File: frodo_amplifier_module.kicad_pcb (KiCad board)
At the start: 2 copper layers, 16.5 x 21.2 mm, 23 parts, among them IC1 INA826AID, IC2 AS321KTR-G1, J1 Conn_01x01_Socket, J2 Conn_01x01_Socket, J3 Conn_01x01_Socket, J4 Conn_01x01_Socket, J5 Conn_01x01_Socket, J6 Conn_01x01_Socket, J7 Conn_01x01_Socket, J8 Conn_01x01_Socket

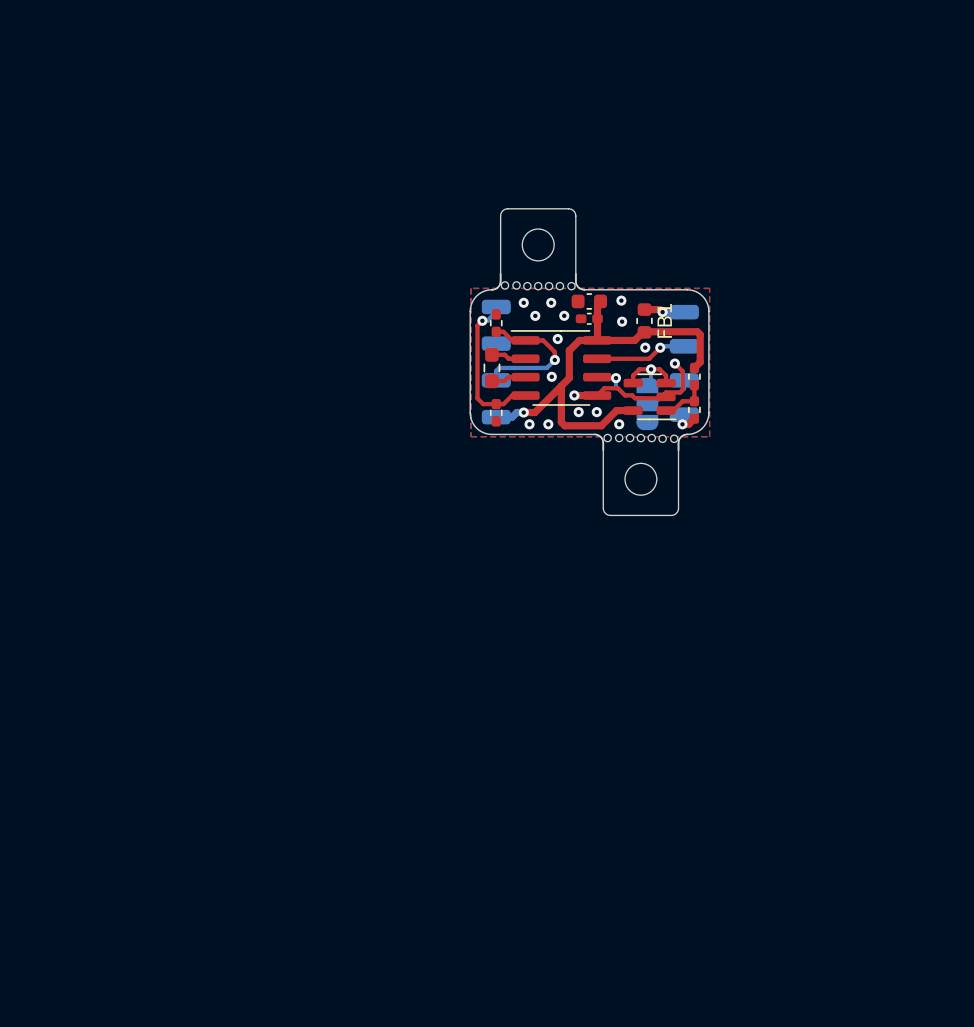
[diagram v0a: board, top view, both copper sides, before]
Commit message: finished the scematics
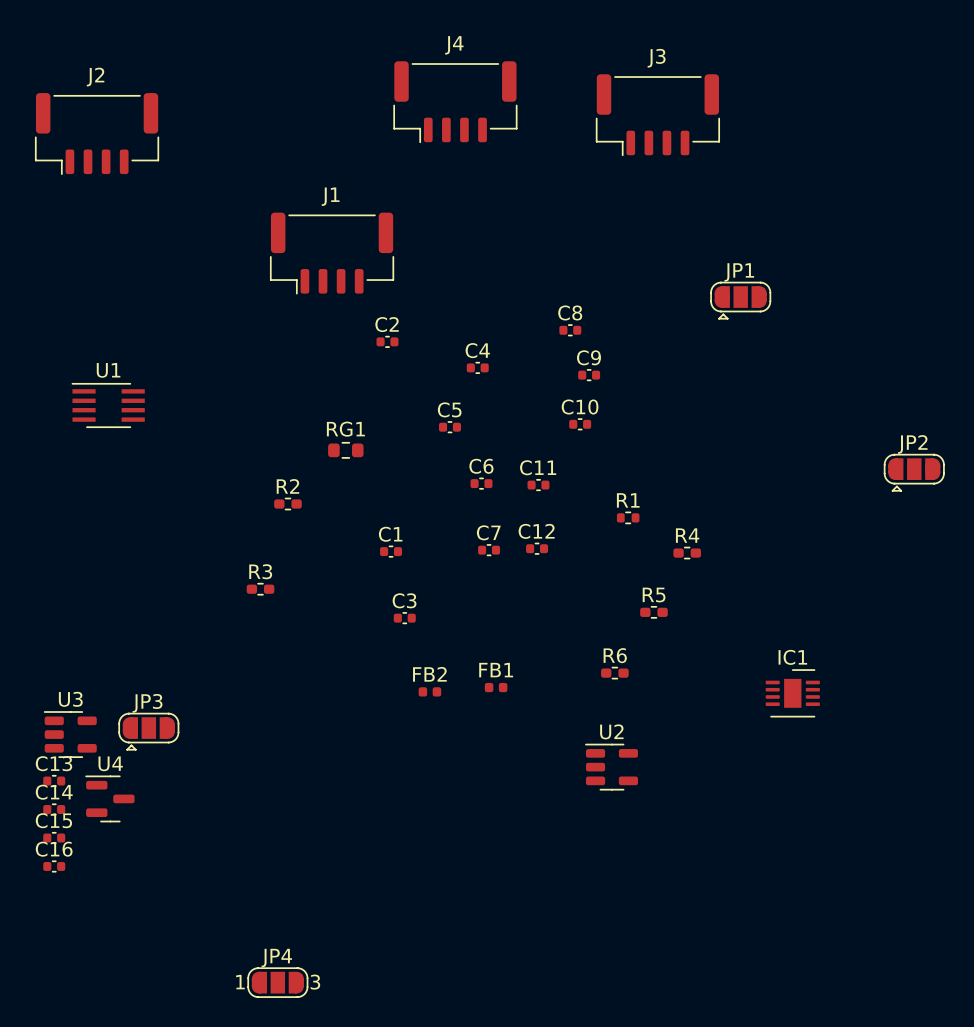
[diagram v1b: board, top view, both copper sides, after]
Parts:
- removed IC2: AS321KTR-G1, Package_TO_SOT_SMD:SOT-23-5
- removed J5, J6, J7, J8: Conn_01x01_Socket, Connector_Wire:SolderWirePad_1x01_SMD_1x2mm
- removed REF** (x2): MountingHole_2.2mm_M2, MountingHole:MountingHole_2.2mm_M2
- removed mouse-bite-2mm-slot (x2): VAL**, MountingEquipment:mouse-bite-2mm-slot
- added C10: 2n2, Capacitor_SMD:C_0402_1005Metric, F.Cu at (80.6, 55.3)
- added C11: 470n, Capacitor_SMD:C_0402_1005Metric, F.Cu at (77.7, 59.5)
- added C12: 0u1, Capacitor_SMD:C_0402_1005Metric, F.Cu at (77.6, 63.9)
- added C13: 0u1, Capacitor_SMD:C_0402_1005Metric, F.Cu at (44.2, 80.0)
- added C14: 0u1, Capacitor_SMD:C_0402_1005Metric, F.Cu at (44.2, 81.9)
- added C15: 1u, Capacitor_SMD:C_0402_1005Metric, F.Cu at (44.2, 83.9)
- added C16: 1u, Capacitor_SMD:C_0402_1005Metric, F.Cu at (44.2, 85.9)
- added C3: 4u7, Capacitor_SMD:C_0402_1005Metric, F.Cu at (68.5, 68.7)
- added C4: 0u1, Capacitor_SMD:C_0402_1005Metric, F.Cu at (73.5, 51.4)
- added C5: 10n, Capacitor_SMD:C_0402_1005Metric, F.Cu at (71.6, 55.5)
- added C6: 2n2, Capacitor_SMD:C_0402_1005Metric, F.Cu at (73.8, 59.4)
- added C7: 10n, Capacitor_SMD:C_0402_1005Metric, F.Cu at (74.3, 64.0)
- added C8: 10n, Capacitor_SMD:C_0402_1005Metric, F.Cu at (79.9, 48.8)
- added C9: 2n2, Capacitor_SMD:C_0402_1005Metric, F.Cu at (81.2, 51.9)
- added FB2: 120R, Inductor_SMD:L_0402_1005Metric, F.Cu at (70.2, 73.8)
- added JP2: SolderJumper_3_Open, Jumper:SolderJumper-3_P1.3mm_Open_RoundedPad1.0x1.5mm, F.Cu at (103.7, 58.4)
- added JP3: SolderJumper_3_Open, Jumper:SolderJumper-3_P1.3mm_Open_RoundedPad1.0x1.5mm, F.Cu at (50.8, 76.3)
- added JP4: SolderJumper_3_Open, Jumper:SolderJumper-3_P1.3mm_Open_RoundedPad1.0x1.5mm_NumberLabels, F.Cu at (59.7, 93.9)
- added R5: 10k, Resistor_SMD:R_0402_1005Metric_Pad0.72x0.64mm_HandSolder, F.Cu at (85.7, 68.3)
- added R6: 10k, Resistor_SMD:R_0402_1005Metric_Pad0.72x0.64mm_HandSolder, F.Cu at (83.0, 72.5)
- added U1: ADC101C021CIMM, Package_SO:SSOP-8_2.95x2.8mm_P0.65mm, F.Cu at (48.0, 54.0)
- added U2: MCP6001-OT, Package_TO_SOT_SMD:SOT-23-5, F.Cu at (82.8, 79.0)
- added U3: MIC5504-3.3YM5, Package_TO_SOT_SMD:SOT-23-5, F.Cu at (45.4, 76.8)
- added U4: REF3033, Package_TO_SOT_SMD:SOT-23, F.Cu at (48.1, 81.2)
- C1: value 100n -> 10u; footprint Capacitor_SMD:C_0402_1005Metric_Pad0.74x0.62mm_HandSolder -> Capacitor_SMD:C_0402_1005Metric
- C2: value 10u -> 100n; footprint Capacitor_SMD:C_0603_1608Metric -> Capacitor_SMD:C_0402_1005Metric
- FB1: footprint Inductor_SMD:L_0603_1608Metric -> Inductor_SMD:L_0402_1005Metric
- IC1: footprint Package_SO:SOIC-8_3.9x4.9mm_P1.27mm -> Package_SON:WSON-8-1EP_3x3mm_P0.5mm_EP1.2x2mm
- J1, J2, J3, J4: value Conn_01x01_Socket -> JST-GH; footprint Connector_Wire:SolderWirePad_1x01_SMD_1x2mm -> Connector_JST:JST_GH_BM04B-GHS-TBT_1x04-1MP_P1.25mm_Vertical; moved to F.Cu
- JP1: footprint Jumper:SolderJumper-3_P1.3mm_Open_RoundedPad1.0x1.5mm_NumberLabels -> Jumper:SolderJumper-3_P1.3mm_Open_RoundedPad1.0x1.5mm; moved to F.Cu
- R1: footprint Resistor_SMD:R_0402_1005Metric_Pad0.72x0.64mm_HandSolder -> Resistor_SMD:R_0402_1005Metric
- R3: value 10k -> 5k
- RG1: footprint Resistor_SMD:R_0603_1608Metric_Pad0.98x0.95mm_HandSolder -> Resistor_SMD:R_0603_1608Metric
- moved J2 43.2 mm to (47.2, 35.2), turned to 0 degrees
- moved R3 33.4 mm to (58.5, 66.7), turned to 0 degrees
- moved IC1 27.6 mm to (95.3, 73.9)
- moved FB1 27.3 mm to (74.8, 73.5), turned to 0 degrees
- moved J4 26.8 mm to (72.0, 33.0), turned to 0 degrees
- moved J1 24.7 mm to (63.4, 43.5), turned to 0 degrees
- moved C1 21.1 mm to (67.5, 64.1), turned to 0 degrees
- moved J3 18.5 mm to (86.0, 33.9), turned to 0 degrees
- moved R1 16.3 mm to (83.9, 61.8), turned to 0 degrees
- moved R2 15.7 mm to (60.4, 60.8), turned to 0 degrees
- moved C2 14.2 mm to (67.3, 49.6), turned to 0 degrees
- moved RG1 11.6 mm to (64.4, 57.1), turned to 0 degrees
- moved R4 9.91 mm to (88.0, 64.2), turned to 0 degrees
- moved JP1 9.82 mm to (91.7, 46.5), turned to 0 degrees
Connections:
- C1 pad 1: VDD -> 5V
- C2 pad 1: VDD -> 3V3
- FB1 pad 1: Net-(J1-Pin_1) -> Net-(J1-Pin_4)
- FB1 pad 2: VDD -> 5V
- IC1 pad 7: out -> sig
- IC1 pad 8: VDD -> 3V3
- J2 pad 1: out -> Net-(J1-Pin_1)
- J3 pad 1: ref -> GND
- JP1 pad 1: GND -> sig2
- JP1 pad 2: ref -> Net-(JP1-C)
- JP1 pad 3: Net-(IC2-INPUT_-) -> sig
- R3 pad 1: Net-(IC2-INPUT_+) -> sig2
- R3 pad 2: VDD -> Net-(J3-Pin_3)
- R4 pad 2: Net-(IC2-INPUT_+) -> sig2
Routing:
- net VDD: track 31.0 -> 0.00 mm, vias 1 -> 0
- net GND: track 11.4 -> 0.00 mm, vias 17 -> 0
- net +IN: track 10.8 -> 0.00 mm, vias 1 -> 0
- net -IN: track 10.2 -> 0.00 mm, vias 1 -> 0
- net ref: track 8.19 -> 0.00 mm, vias 1 -> 0
- net out: track 6.38 -> 0.00 mm, vias 1 -> 0
- net Net-(IC2-INPUT_-): track 4.99 -> 0.00 mm, vias 1 -> 0
- net Net-(IC2-INPUT_+): track 3.28 -> 0.00 mm
- net Net-(J1-Pin_1): track 2.82 -> 0.00 mm, vias 1 -> 0
- net Net-(IC1-RG_2): track 2.44 -> 0.00 mm
- net Net-(IC1-RG_1): track 2.44 -> 0.00 mm
- removed copper zone on B.Cu, net GND
- removed copper zone on F.Cu, net GND
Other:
- board outline removed
- copper layers 2 -> 4
- board text removed: "1 gnd"
- board text removed: "3 ref"
- board text removed: "<io sens>"
- board text removed: "JLCJLCJLCJLC"
- board text removed: "o+"
- board text removed: "ref"
- board text removed: "s+"
- board text removed: "s-"
- board text removed: "u+"
- board text removed: "u-"
